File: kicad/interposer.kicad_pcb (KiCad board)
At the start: 2 copper layers, 22.9 x 26.7 mm, 9 parts, among them J1 Conn_Stove, U1 XIAO-nRF52840, U2 Adafruit DS3502, U3 TS5A3159DBV

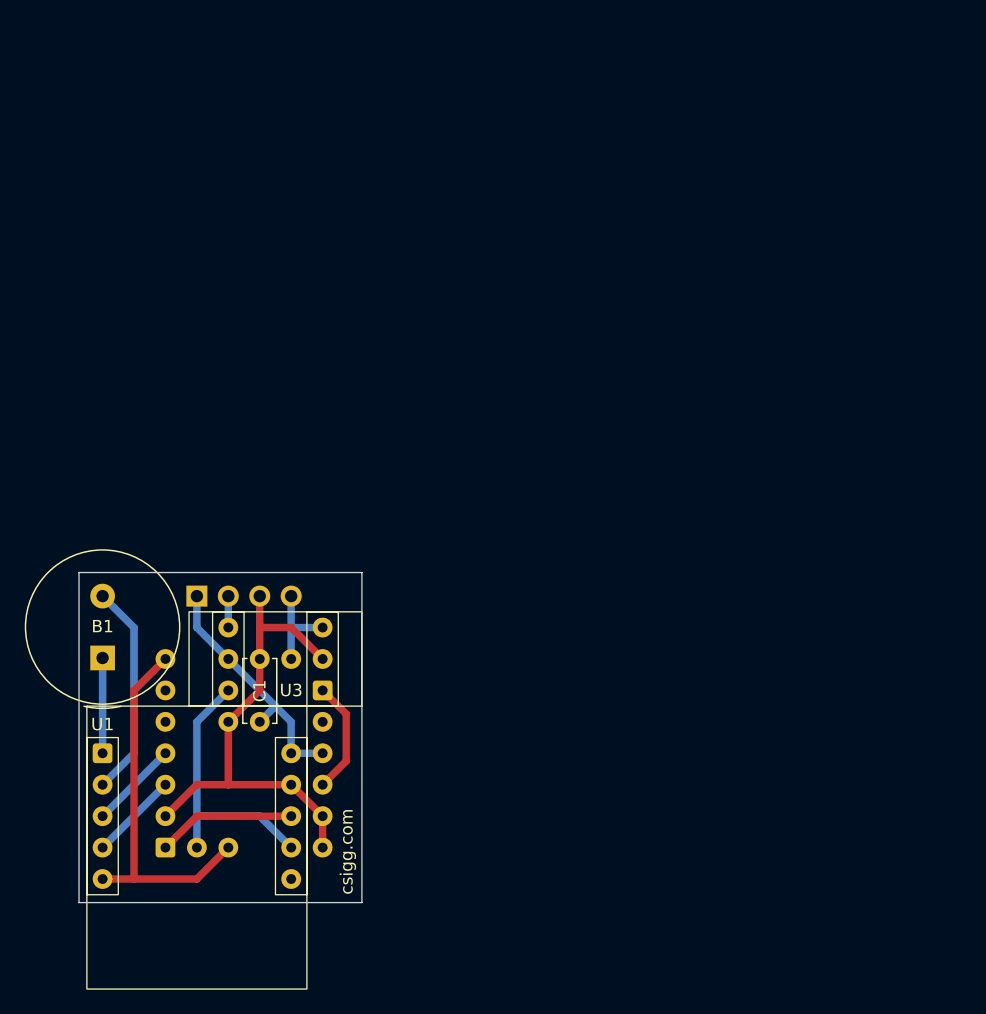
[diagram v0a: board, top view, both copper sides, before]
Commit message: Update KiCad
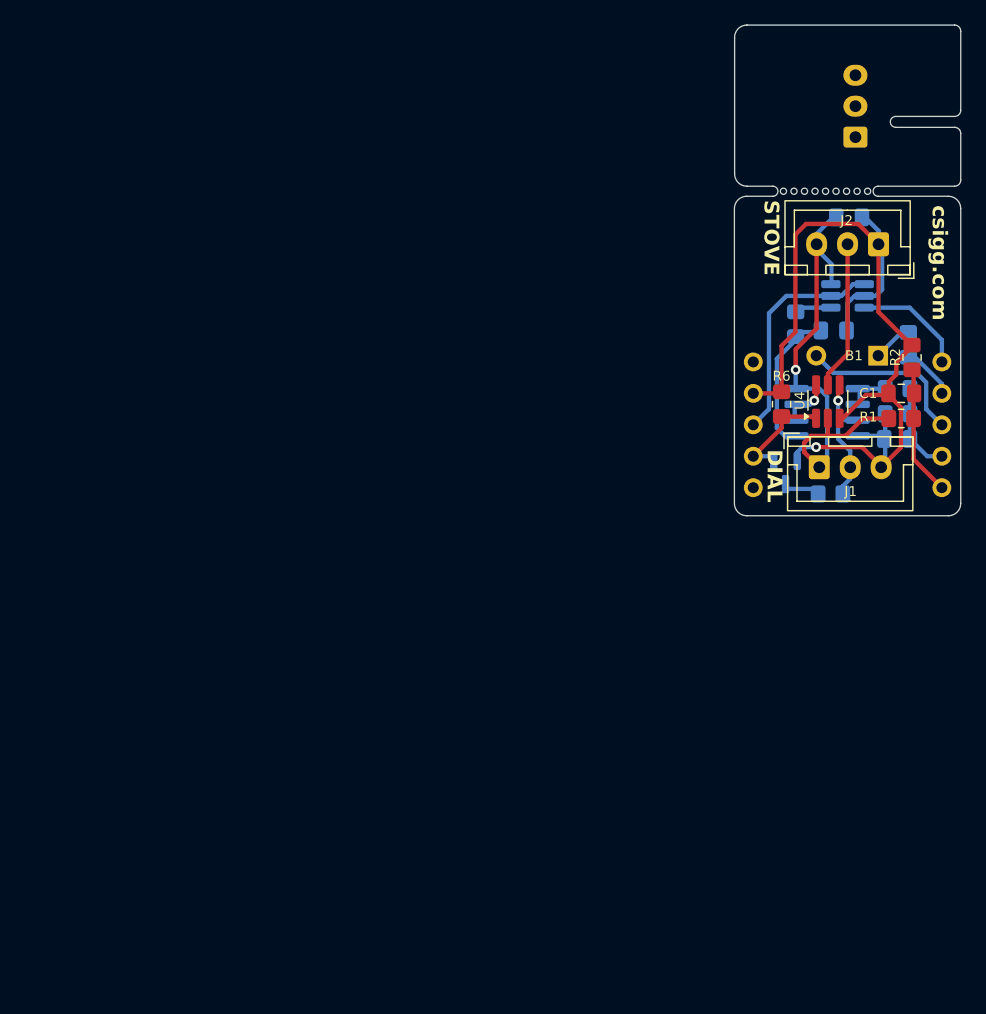
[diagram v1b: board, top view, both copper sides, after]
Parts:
- added C2: 100nF, Capacitor_SMD:C_0805_2012Metric_Pad1.18x1.45mm_HandSolder, B.Cu at (127.7, 88.9)
- added C3: 1µF, Capacitor_SMD:C_0805_2012Metric_Pad1.18x1.45mm_HandSolder, B.Cu at (122.6, 80.1)
- added C4: 1µF, Capacitor_SMD:C_0805_2012Metric_Pad1.18x1.45mm_HandSolder, B.Cu at (123.8, 71.0)
- added J2: Stove, Connector_JST:JST_XH_B3B-XH-A_1x03_P2.50mm_Vertical, F.Cu at (126.2, 73.2)
- added J3: Stove, Connector_JST:JST_XH_S3B-XH-A_1x03_P2.50mm_Horizontal, B.Cu at (124.3, 64.5)
- added Q1: 2N7002, Package_TO_SOT_SMD:SOT-23, B.Cu at (118.7, 91.6)
- added R4: 51kΩ, Resistor_SMD:R_0805_2012Metric_Pad1.20x1.40mm_HandSolder, B.Cu at (127.7, 86.9)
- added R5: 33kΩ, Resistor_SMD:R_0805_2012Metric_Pad1.20x1.40mm_HandSolder, B.Cu at (119.5, 79.6)
- added R6: 100kΩ, Resistor_SMD:R_0805_2012Metric_Pad1.20x1.40mm_HandSolder, F.Cu at (118.4, 86.1)
- added R7: 100Ω, Resistor_SMD:R_0805_2012Metric_Pad1.20x1.40mm_HandSolder, B.Cu at (128.6, 81.3)
- added R8: 1MΩ, Resistor_SMD:R_0805_2012Metric_Pad1.20x1.40mm_HandSolder, B.Cu at (122.3, 93.3)
- added REF**: BreakLine_9h_D0.5mm_P0.85mm, Panelization:BreakLine_9h_D0.5mm_P0.85mm, F.Cu at (121.9, 68.9)
- added U4: TMUX1119DBVR, Package_TO_SOT_SMD:SOT-23-6_Handsoldering, F.Cu at (122.1, 85.9)
- B1: footprint Buzzer_Beeper:Buzzer_TDK_PS1240P02BT_D12.2mm_H6.5mm -> interposer:Buzzer_TDK_PS1240P02BT_D12.2mm_H6.5mm
- C1: value 0.1µF -> 100nF; footprint Capacitor_THT:C_Disc_D5.0mm_W2.5mm_P5.00mm -> Capacitor_SMD:C_0805_2012Metric_Pad1.18x1.45mm_HandSolder
- J1: value Conn_Stove -> Dial; footprint Connector_PinHeader_2.54mm:PinHeader_1x04_P2.54mm_Vertical -> Connector_JST:JST_XH_B3B-XH-A_1x03_P2.50mm_Vertical; moved to F.Cu
- R1: value 10kΩ -> 27kΩ; footprint Resistor_THT:R_Axial_DIN0207_L6.3mm_D2.5mm_P10.16mm_Horizontal -> Resistor_SMD:R_0805_2012Metric_Pad1.20x1.40mm_HandSolder; moved to F.Cu
- R2: value 18kΩ -> 51kΩ; footprint Resistor_THT:R_Axial_DIN0207_L6.3mm_D2.5mm_P10.16mm_Horizontal -> Resistor_SMD:R_0805_2012Metric_Pad1.20x1.40mm_HandSolder; moved to F.Cu
- R3: value 10kΩ -> 27kΩ; footprint Resistor_THT:R_Axial_DIN0207_L6.3mm_D2.5mm_P10.16mm_Horizontal -> Resistor_SMD:R_0805_2012Metric_Pad1.20x1.40mm_HandSolder
- U1: value XIAO-nRF52840 -> XIAO-nRF52840-DIP; footprint Package_DIP:DIP-14_W7.62mm -> interposer:XIAO-nRF52840-DIP; moved to B.Cu
- U2: value Adafruit DS3502 -> MCP6042-E_SN; footprint Package_DIP:DIP-12_W7.62mm -> Package_SO:SOIC-8_3.9x4.9mm_P1.27mm
- U3: value TS5A3159DBV -> TXU0101DBVR; footprint Package_DIP:DIP-6_W7.62mm -> Package_TO_SOT_SMD:SOT-23-6_Handsoldering; moved to B.Cu
- moved R2 68.0 mm to (128.9, 82.3)
- moved R3 67.7 mm to (127.7, 84.8)
- moved B1 67.3 mm to (126.2, 82.2), turned to 180 degrees
- moved U1 64.8 mm to (123.7, 90.3), turned to 90 degrees
- moved U2 64.0 mm to (122.0, 86.7), turned to 180 degrees
- moved C1 58.2 mm to (128.0, 85.2), turned to 180 degrees
- moved U3 53.1 mm to (123.7, 77.3)
- moved R1 53.0 mm to (128.0, 87.2), turned to 0 degrees
- moved J1 51.4 mm to (121.4, 91.2), turned to 0 degrees
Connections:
- B1 pad 1: Net-(U1-PA02_A0_D0) -> Net-(B1-Pad1)
- B1 pad 2: Net-(U1-PA4_A1_D1) -> /-BUZZ
- C1 pad 1: +5V -> /REF
- J1 pad 2: /RETURN -> /DIAL
- R1 pad 1: /KNOB -> +5V
- R1 pad 2: /INPUT -> /REF
- R2 pad 1: /INPUT -> /REF
- R3 pad 1: /BYPASS -> /IN
- R3 pad 2: GND -> /READ
- U1 pad 1: Net-(U1-PA02_A0_D0) -> /PWM_3V3
- U1 pad 11: /BYPASS -> /SEL
- U1 pad 14: +5V -> unconnected-(U1-VBUS-Pad14)
- U1 pad 2: Net-(U1-PA4_A1_D1) -> /+BUZZ
- U1 pad 3: /SCL -> /-BUZZ
- U1 pad 4: /SDA -> /READ
- U1 pad 5: /INPUT -> /REF
- U2 pad 1: /SCL -> /IN
- U2 pad 2: GND -> /IN
- U2 pad 3: +3V3 -> /DIAL
- U2 pad 4: unconnected-(U2-A1-Pad4) -> GND
- U2 pad 5: unconnected-(U2-A0-Pad5) -> /RC
- U2 pad 6: +5V -> /OUT
- U2 pad 7: /OUPUT -> /OUT
- U2 pad 8: GND -> +5V
- U3 pad 1: /OUPUT -> +3V3
- U3 pad 3: /KNOB -> /PWM_3V3
- U3 pad 4: /RETURN -> /PWM_5V
- U3 pad 5: +5V -> +3V3
- U3 pad 6: /BYPASS -> +5V
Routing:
- net GND: track 39.8 -> 74.0 mm, vias 0 -> 1
- net /INPUT: track 30.0 -> 0.00 mm
- net /BYPASS: track 22.4 -> 0.00 mm
- net +5V: track 20.2 -> 39.1 mm, vias 0 -> 1
- net Net-(U1-PA4_A1_D1): track 17.3 -> 0.00 mm
- net /-BUZZ: track 0.00 -> 13.7 mm
- net /STOVE: track 0.00 -> 12.7 mm
- net /DIAL: track 0.00 -> 11.1 mm, vias 0 -> 1
- net /RC: track 0.00 -> 11.1 mm
- net /REF: track 0.00 -> 10.5 mm
- net /OUPUT: track 9.20 -> 0.00 mm
- net /PWM_3V3: track 0.00 -> 9.18 mm
- net /SEL: track 0.00 -> 8.65 mm
- net Net-(U1-PA02_A0_D0): track 7.70 -> 0.00 mm
- net /KNOB: track 7.62 -> 0.00 mm
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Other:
- board size 22.9 x 26.7 mm -> 18.3 x 39.7 mm
- board text added: "Conn_Internal"
- board text added: "DIAL"
- board text added: "STOVE"
